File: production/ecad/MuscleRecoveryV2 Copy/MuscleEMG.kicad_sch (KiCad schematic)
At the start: 41 parts, among them J1 AudioJack3, J2 Screw_Terminal_01x03, J5 Screw_Terminal_01x10, U5 AD8232ACPZ-R7, U7 ADS1115IDGS

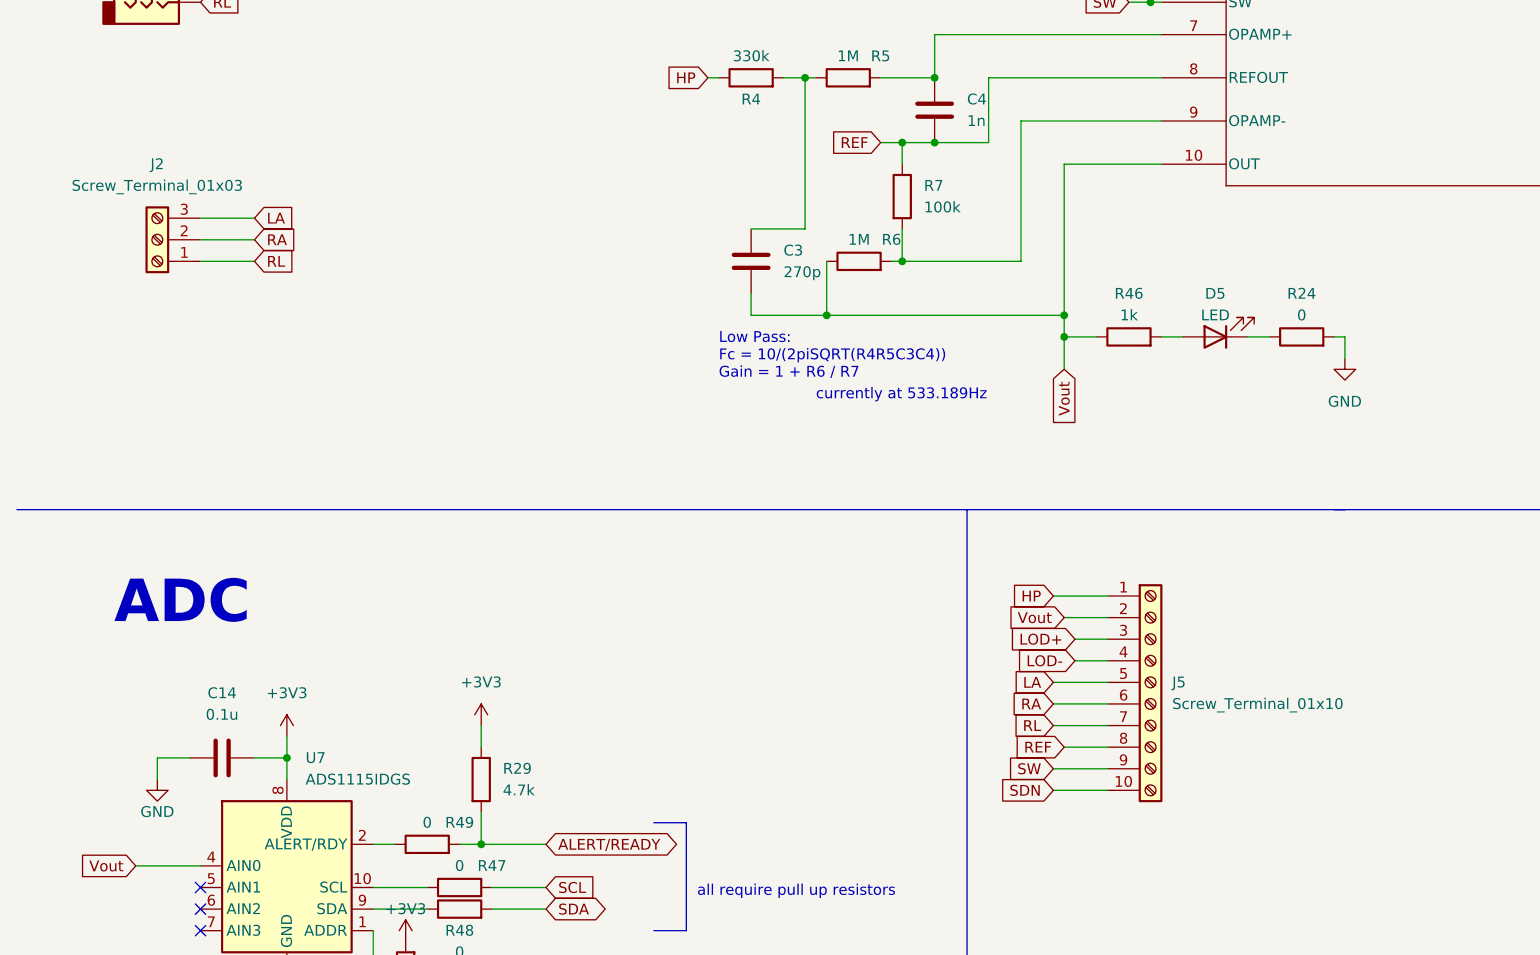
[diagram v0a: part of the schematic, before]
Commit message: Created New Layout
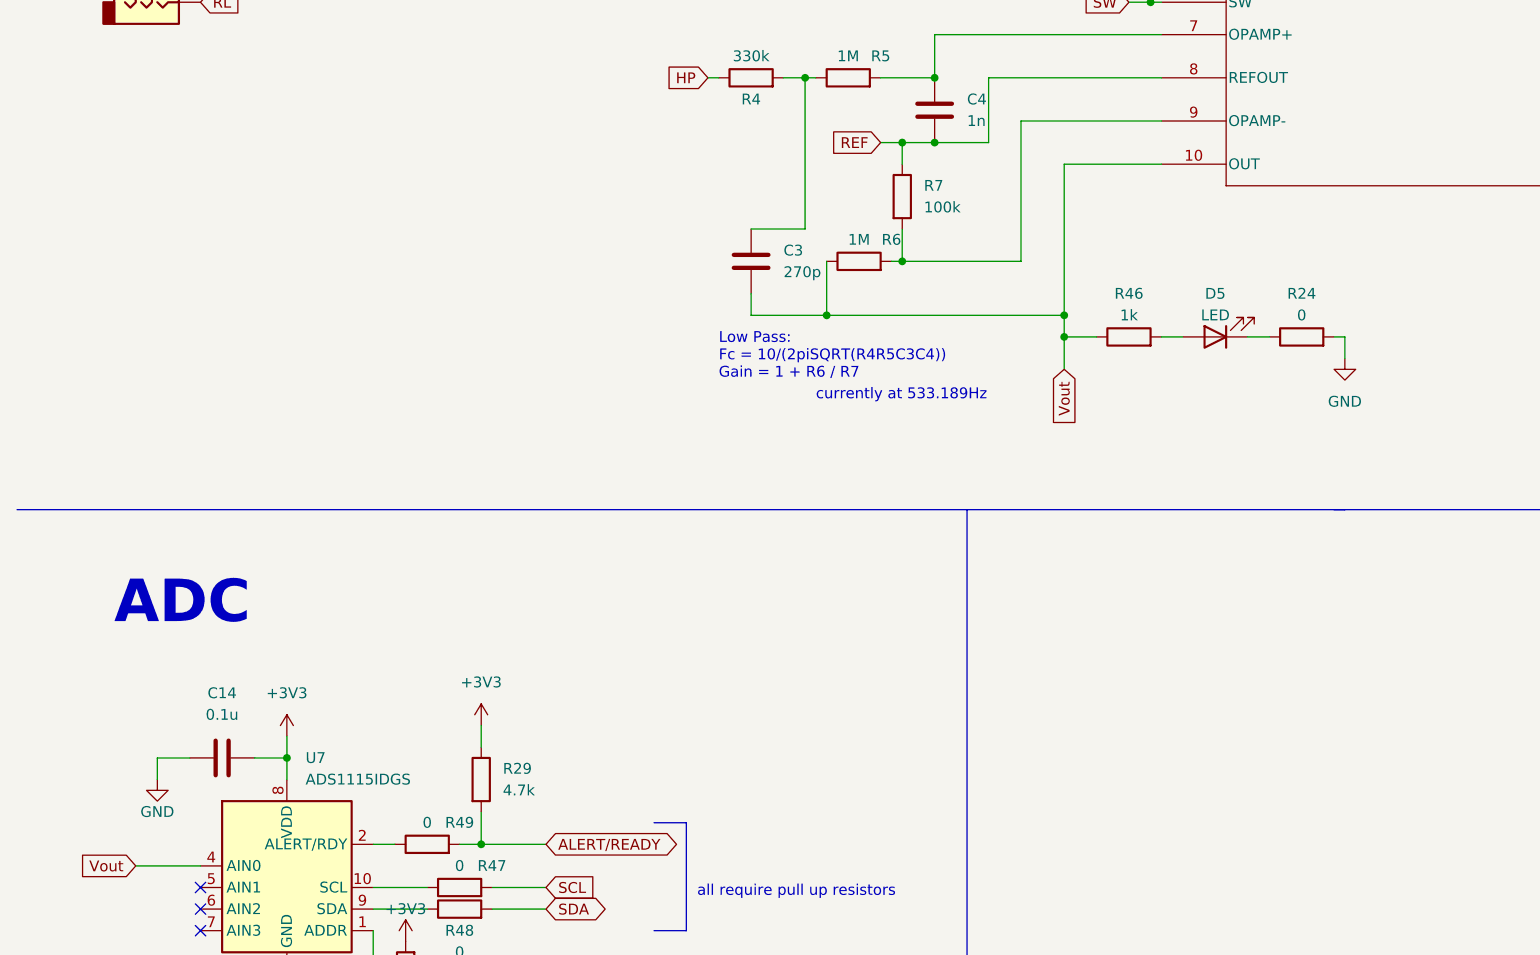
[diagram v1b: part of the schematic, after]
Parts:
- removed J2: Screw_Terminal_01x03, symbol Connector:Screw_Terminal_01x03
- removed J5: Screw_Terminal_01x10, symbol Connector:Screw_Terminal_01x10
- C1, C10, C11, C14, C2, C3, C4: footprint Capacitor_SMD:C_0805_2012Metric -> Capacitor_SMD:C_0402_1005Metric
- D5, D6: footprint LED_THT:LED_D1.8mm_W3.3mm_H2.4mm -> LED_SMD:LED_0402_1005Metric
- J1: footprint (none) -> Muscle_Recovery_Footprint_Library:CUI_SJ-3523-SMT-TR
- R1, R19, R2, R20, R21, R22, R23, R24, R25, R26, R28, R29, R3, R4, R5, R6, R61, R62, R63, R64, R7: footprint Resistor_SMD:R_0805_2012Metric -> Resistor_SMD:R_0402_1005Metric
- R44, R45, R46, R47, R48, R49: footprint Resistor_SMD:R_0805_2012Metric -> Resistor_SMD:R_01005_0402Metric
- U5: footprint AD8232ACPZ-R7:CP_20_10_ADI -> Muscle_Recovery_Footprint_Library:LFCSP_20

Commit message: Pushing Layout Changes for Andy's Layout
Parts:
- R44, R45, R46, R47, R48, R49: footprint Resistor_SMD:R_01005_0402Metric -> Resistor_SMD:R_0402_1005Metric
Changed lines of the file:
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@@
       (effects (font (size 1.27 1.27)))
     )
-    (property "Footprint" "Resistor_SMD:R_01005_0402Metric" (at 66.04 171.958 90)
+    (property "Footprint" "Resistor_SMD:R_0402_1005Metric" (at 66.04 171.958 90)
       (effects (font (size 1.27 1.27)) hide)
     )
@@
       (effects (font (size 1.27 1.27)))
     )
-    (property "Footprint" "Resistor_SMD:R_01005_0402Metric" (at 138.43 24.638 90)
+    (property "Footprint" "Resistor_SMD:R_0402_1005Metric" (at 138.43 24.638 90)
       (effects (font (size 1.27 1.27)) hide)
     )
@@
       (effects (font (size 1.27 1.27)))
     )
-    (property "Footprint" "Resistor_SMD:R_01005_0402Metric" (at 121.92 24.638 90)
+    (property "Footprint" "Resistor_SMD:R_0402_1005Metric" (at 121.92 24.638 90)
       (effects (font (size 1.27 1.27)) hide)
     )
@@
       (effects (font (size 1.27 1.27)))
     )
-    (property "Footprint" "Resistor_SMD:R_01005_0402Metric" (at 66.04 174.498 90)
+    (property "Footprint" "Resistor_SMD:R_0402_1005Metric" (at 66.04 174.498 90)
       (effects (font (size 1.27 1.27)) hide)
     )
@@
       (effects (font (size 1.27 1.27)))
     )
-    (property "Footprint" "Resistor_SMD:R_01005_0402Metric" (at 144.78 107.188 90)
+    (property "Footprint" "Resistor_SMD:R_0402_1005Metric" (at 144.78 107.188 90)
       (effects (font (size 1.27 1.27)) hide)
     )
@@
       (effects (font (size 1.27 1.27)))
     )
-    (property "Footprint" "Resistor_SMD:R_01005_0402Metric" (at 62.23 166.878 90)
-      (effects (font (size 1.27 1.27)) hide)
-    )
+    (property "Footprint" "Resistor_SMD:R_0402_1005Metric" (at 62.23 166.878 90)
+      (effects (font (size 1.27 1.27)) hide)
+    )

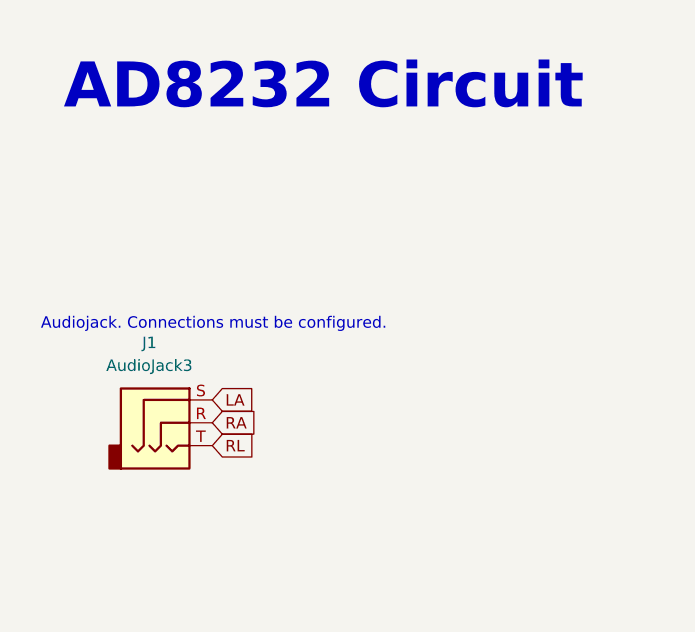
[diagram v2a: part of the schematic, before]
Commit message: Committing My pliminary placement for my PCB <3
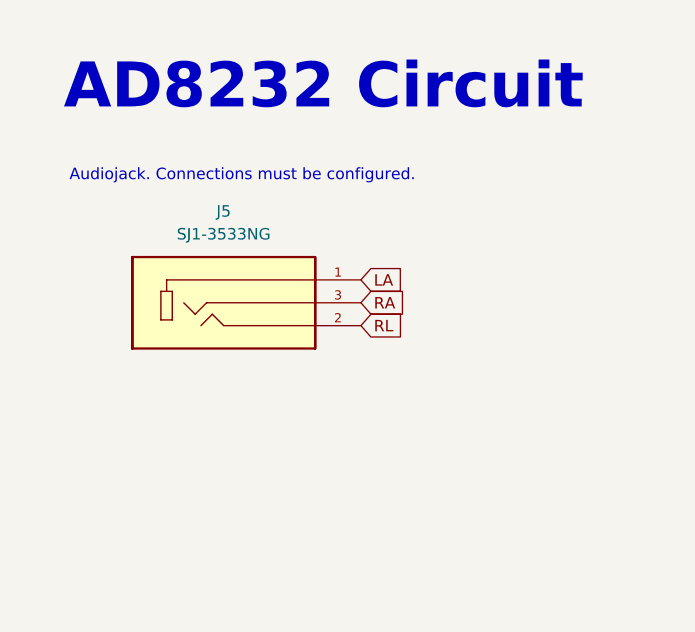
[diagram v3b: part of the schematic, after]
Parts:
- removed J1: AudioJack3, Muscle_Recovery_Footprint_Library:CUI_SJ-3523-SMT-TR, symbol Connector_Audio:AudioJack3
- added J5: SJ1-3533NG, Muscle_Recovery_Footprint_Library:CUI_SJ1-3533NG, symbol MuscleRecoverySymbolLibray:SJ1-3533NG
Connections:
- net LA: now also J5.1
- net RA: now also J5.3
- net RL: now also J5.2
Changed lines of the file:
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@@
     (effects (font (size 1.27 1.27)) (justify left bottom))
   )
-  (text "Audiojack. Connections must be configured." (at 16.51 53.34 0)
+  (text "Audiojack. Connections must be configured." (at 19.685 36.83 0)
     (effects (font (size 1.27 1.27)) (justify left bottom))
   )
@@
     (effects (font (size 5 5) bold) (justify left bottom))
   )
-  (global_label "RA" (shape input) (at 35.56 63.5 0) (fields_autoplaced)
-    (effects (font (size 1.27 1.27)) (justify left))
-    (property "Intersheetrefs" "${INTERSHEET_REFS}" (at 40.9038 63.5 0)
+  (global_label "RA" (shape input) (at 52.07 50.165 0) (fields_autoplaced)
+    (effects (font (size 1.27 1.27)) (justify left))
+    (property "Intersheetrefs" "${INTERSHEET_REFS}" (at 57.4138 50.165 0)
       (effects (font (size 1.27 1.27)) (justify left) hide)
     )
@@
     )
   )
-  (global_label "RL" (shape input) (at 35.56 66.04 0) (fields_autoplaced)
-    (effects (font (size 1.27 1.27)) (justify left))
-    (property "Intersheetrefs" "${INTERSHEET_REFS}" (at 40.8433 66.04 0)
+  (global_label "RL" (shape input) (at 52.07 52.705 0) (fields_autoplaced)
+    (effects (font (size 1.27 1.27)) (justify left))
+    (property "Intersheetrefs" "${INTERSHEET_REFS}" (at 57.3533 52.705 0)
       (effects (font (size 1.27 1.27)) (justify left) hide)
     )
@@
     )
   )
-  (global_label "LA" (shape input) (at 35.56 60.96 0) (fields_autoplaced)
-    (effects (font (size 1.27 1.27)) (justify left))
-    (property "Intersheetrefs" "${INTERSHEET_REFS}" (at 40.6619 60.96 0)
+  (global_label "LA" (shape input) (at 52.07 47.625 0) (fields_autoplaced)
+    (effects (font (size 1.27 1.27)) (justify left))
+    (property "Intersheetrefs" "${INTERSHEET_REFS}" (at 57.1719 47.625 0)
       (effects (font (size 1.27 1.27)) (justify left) hide)
     )
@@
     )
   )
+  (symbol (lib_id "MuscleRecoverySymbolLibray:SJ1-3533NG") (at 36.83 50.165 0) (unit 1)
+    (in_bom yes) (on_board yes) (dnp no) (fields_autoplaced)
+    (property "Reference" "J5" (at 36.83 40.005 0)
+      (effects (font (size 1.27 1.27)))
+    )
+    (property "Value" "SJ1-3533NG" (at 36.83 42.545 0)
+      (effects (font (size 1.27 1.27)))
+    )
+    (property "Footprint" "Muscle_Recovery_Footprint_Library:CUI_SJ1-3533NG" (at 36.83 50.165 0)
+      (effects (font (size 1.27 1.27)) (justify left bottom) hide)
+    )
+    (property "Datasheet" "" (at 36.83 50.165 0)
+      (effects (font (size 1.27 1.27)) (justify left bottom) hide)
+    )
+    (property "MF" "CUI Devices" (at 36.83 50.165 0)
+      (effects (font (size 1.27 1.27)) (justify left bottom) hide)
+    )
+    (property "DESCRIPTION" "3.5 mm, Stereo, Right Angle, Through Hole, Isolated Ground, Audio Jack Connector" (at 36.83 50.165 0)
+      (effects (font (size 1.27 1.27)) (justify left bottom) hide)
+    )
+    (property "PACKAGE" "None" (at 36.83 50.165 0)
+      (effects (font (size 1.27 1.27)) (justify left bottom) hide)
+    )
+    (property "PRICE" "None" (at 36.83 50.165 0)
+      (effects (font (size 1.27 1.27)) (justify left bottom) hide)
+    )
+    (property "CUI_PURCHASE_URL" "https://www.cuidevices.com/product/interconnect/connectors/audio-connectors/jacks/sj1-353xng-series?utm_source=snapeda.com&utm_medium=referral&utm_campaign=snapedaBOM" (at 36.83 50.165 0)
+      (effects (font (size 1.27 1.27)) (justify left bottom) hide)
+    )
+    (property "MP" "SJ1-3533NG" (at 36.83 50.165 0)
+      (effects (font (size 1.27 1.27)) (justify left bottom) hide)
+    )
+    (property "AVAILABILITY" "Unavailable" (at 36.83 50.165 0)
+      (effects (font (size 1.27 1.27)) (justify left bottom) hide)
+    )
+    (pin "1")
+    (pin "2")
+    (pin "3")
+    (instances
+      (project "MuscleRecoveryV1"
+        (path "/4e550305-79d2-4e4a-a502-817ebcc79f9a/284c60dd-e199-4b03-b99f-cc7eaed256f8"
+          (reference "J5") (unit 1)
+        )
+      )
+    )
+  )
   (symbol (lib_id "Analog_ADC:ADS1115IDGS") (at 45.72 170.18 0) (unit 1)
     (in_bom yes) (on_board yes) (dnp no) (fields_autoplaced)
@@
         )
       )
-    )
-  )
-  (symbol (lib_id "Connector_Audio:AudioJack3") (at 30.48 63.5 0) (unit 1)
-    (in_bom yes) (on_board yes) (dnp no) (fields_autoplaced)
-    (property "Reference" "J1" (at 28.575 54.61 0)
-      (effects (font (size 1.27 1.27)))
-    )
-    (property "Value" "AudioJack3" (at 28.575 57.15 0)
-      (effects (font (size 1.27 1.27)))
-    )
-    (property "Footprint" "Muscle_Recovery_Footprint_Library:CUI_SJ-3523-SMT-TR" (at 30.48 63.5 0)
-      (effects (font (size 1.27 1.27)) hide)
-    )
-    (property "Datasheet" "~" (at 30.48 63.5 0)
-      (effects (font (size 1.27 1.27)) hide)
-    )
-    (pin "R")
-    (pin "S")
-    (pin "T")
-    (instances
-      (project "MuscleRecoveryV1"
-        (path "/4e550305-79d2-4e4a-a502-817ebcc79f9a/284c60dd-e199-4b03-b99f-cc7eaed256f8"
-          (reference "J1") (unit 1)
-        )
-      )
